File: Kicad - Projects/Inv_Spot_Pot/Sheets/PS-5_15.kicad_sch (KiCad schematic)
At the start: 23 parts, among them U2 LTV-817S

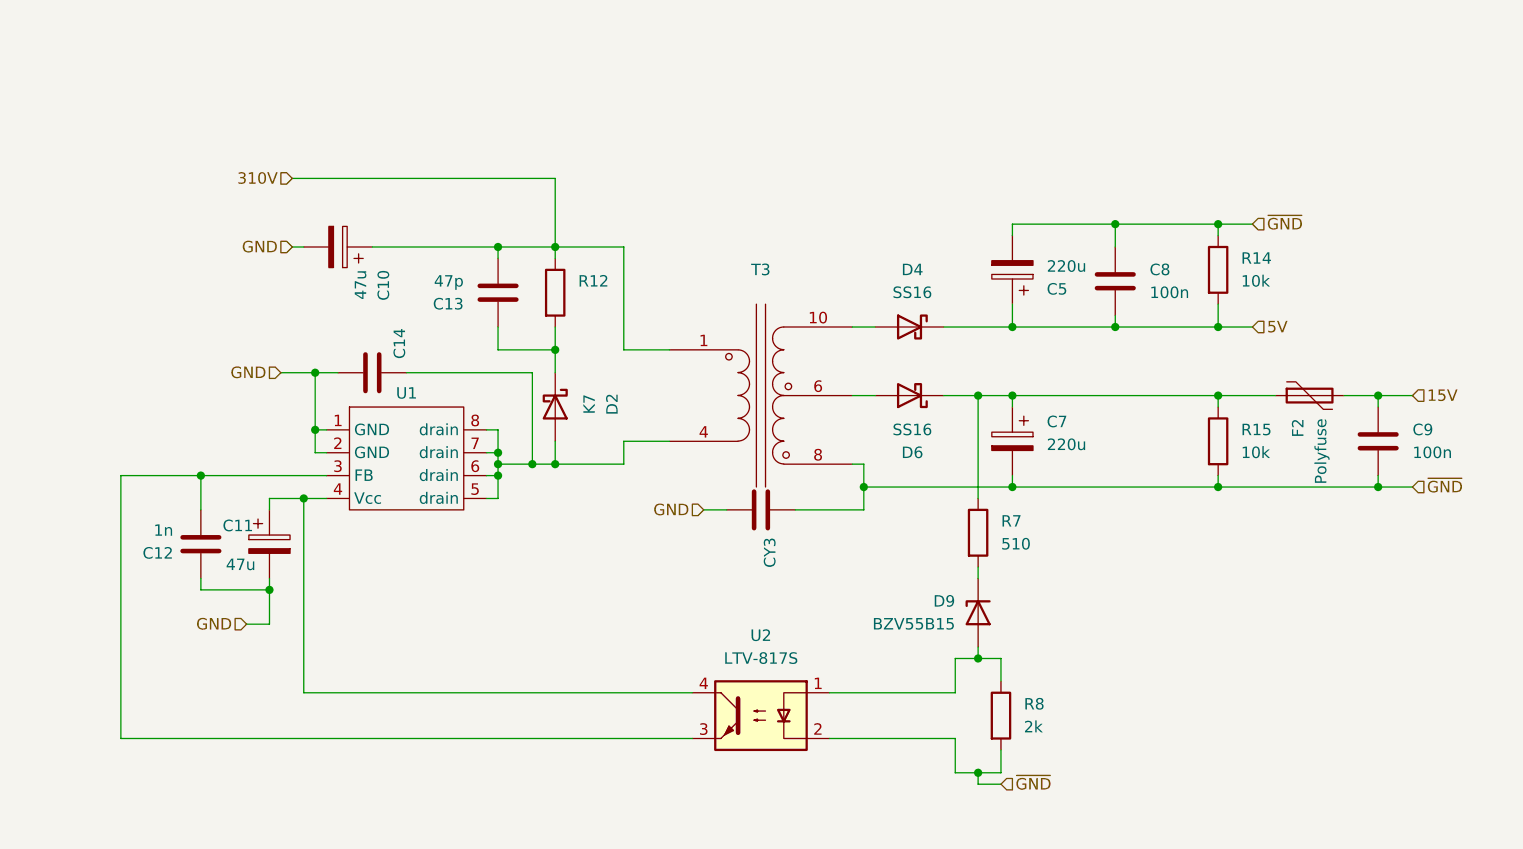
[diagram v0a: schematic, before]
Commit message: Adicionado Footprint do Transformador
Footprint do transformador adicionada

Linha dos capacitores XY adicionada

Alteração nas linhas de PWM
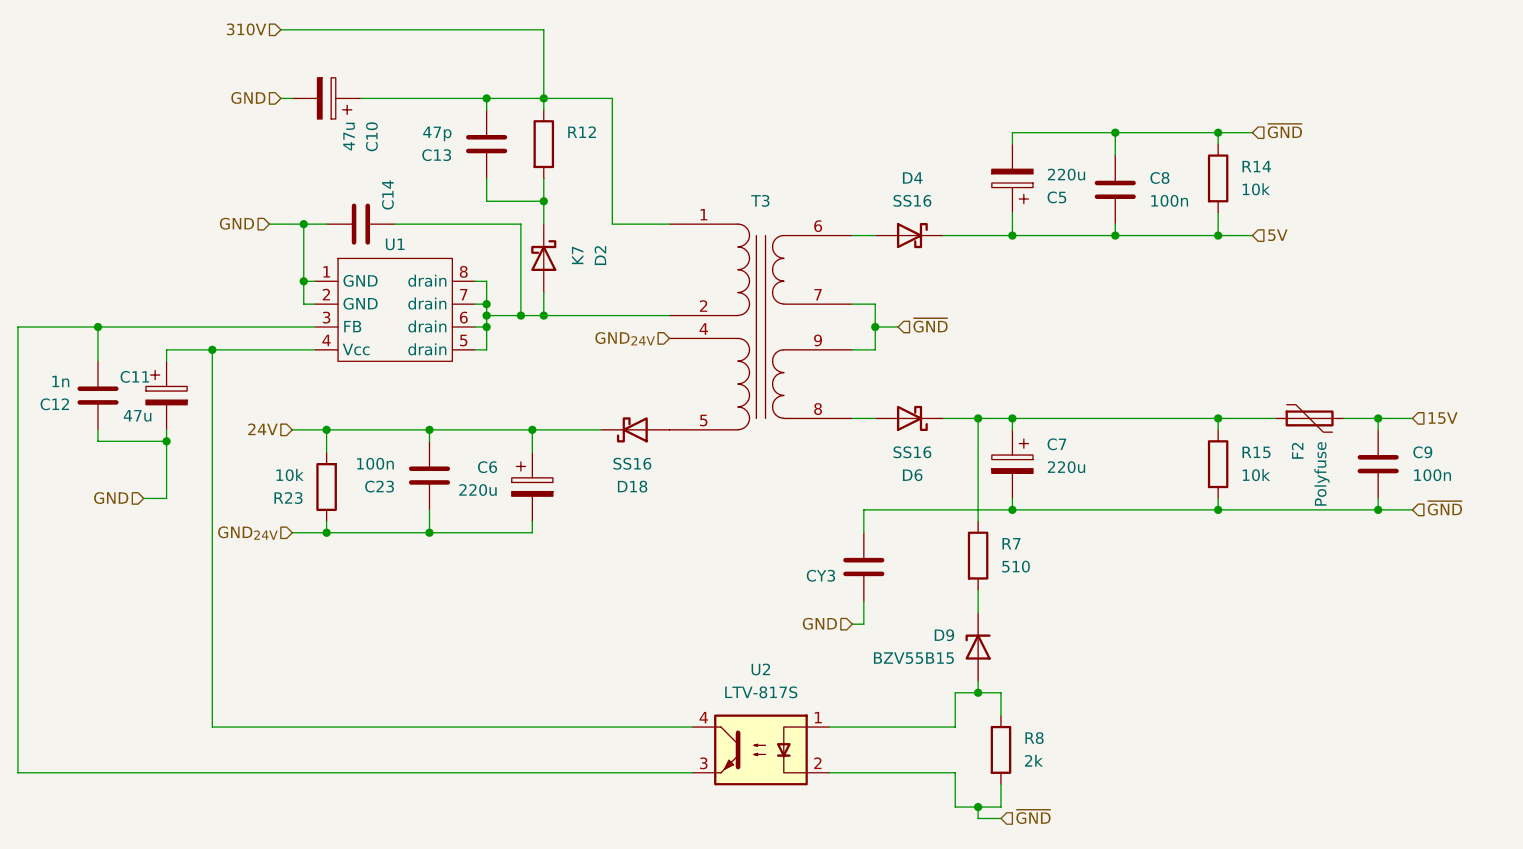
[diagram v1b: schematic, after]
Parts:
- removed T3: (no value), Transformer_THT:Custom_Transformer-10P-EEL22_EE30_7, symbol Custom_Transformers:Transformer_1P_2S_CT
- added C23: 100n, Capacitor_SMD:C_1206_3216Metric_Pad1.33x1.80mm_HandSolder, symbol Device:C
- added C6: 220u, Capacitor_THT:CP_Radial_D8.0mm_P3.50mm, symbol Device:C_Polarized
- added D18: SS16, Diode_SMD:D_SOD-128, symbol Device:D_Schottky
- added R23: 10k, Resistor_SMD:R_1206_3216Metric_Pad1.30x1.75mm_HandSolder, symbol Device:R
- added T3: (no value), Transformer_THT:Transformer_Breve_TEZ-28x33, symbol Custom_Transformers:Transformer_1P_3S_CT
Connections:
- net 310V: now also T3.1
- net GND: now also CY3.2; no longer CY3.1
- net ~{GND}: now also CY3.1, T3.7, T3.9; no longer CY3.2
- net at C14.2, D2.2 (A), U1.5 (drain)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: now also T3.2
- net at D4.2 (A): now also T3.6
- net at D6.2 (A): now also T3.8
- new net: D18.2 (A), T3.5
- new net 24V: C23.2, C6.1, D18.1 (K), R23.2
- new net GND_{24V}: C23.1, C6.2, R23.1, T3.4
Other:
- moved on the sheet: C10, C11, C12, C13, C14, C5, C7, C8, C9, CY3, D2, D4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
